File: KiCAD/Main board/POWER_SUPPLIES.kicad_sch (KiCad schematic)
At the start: 30 parts, among them U18 12V, U19 5V, U20 8V, U21 15V, U23 LIN_REG_±5V, U24 LIN_REG_±12V, U28 12V, U29 AP2111H-3.3TRG1, U31 AP2111H-3.3TRG1, U9 SEPIC_-15V_LT3579

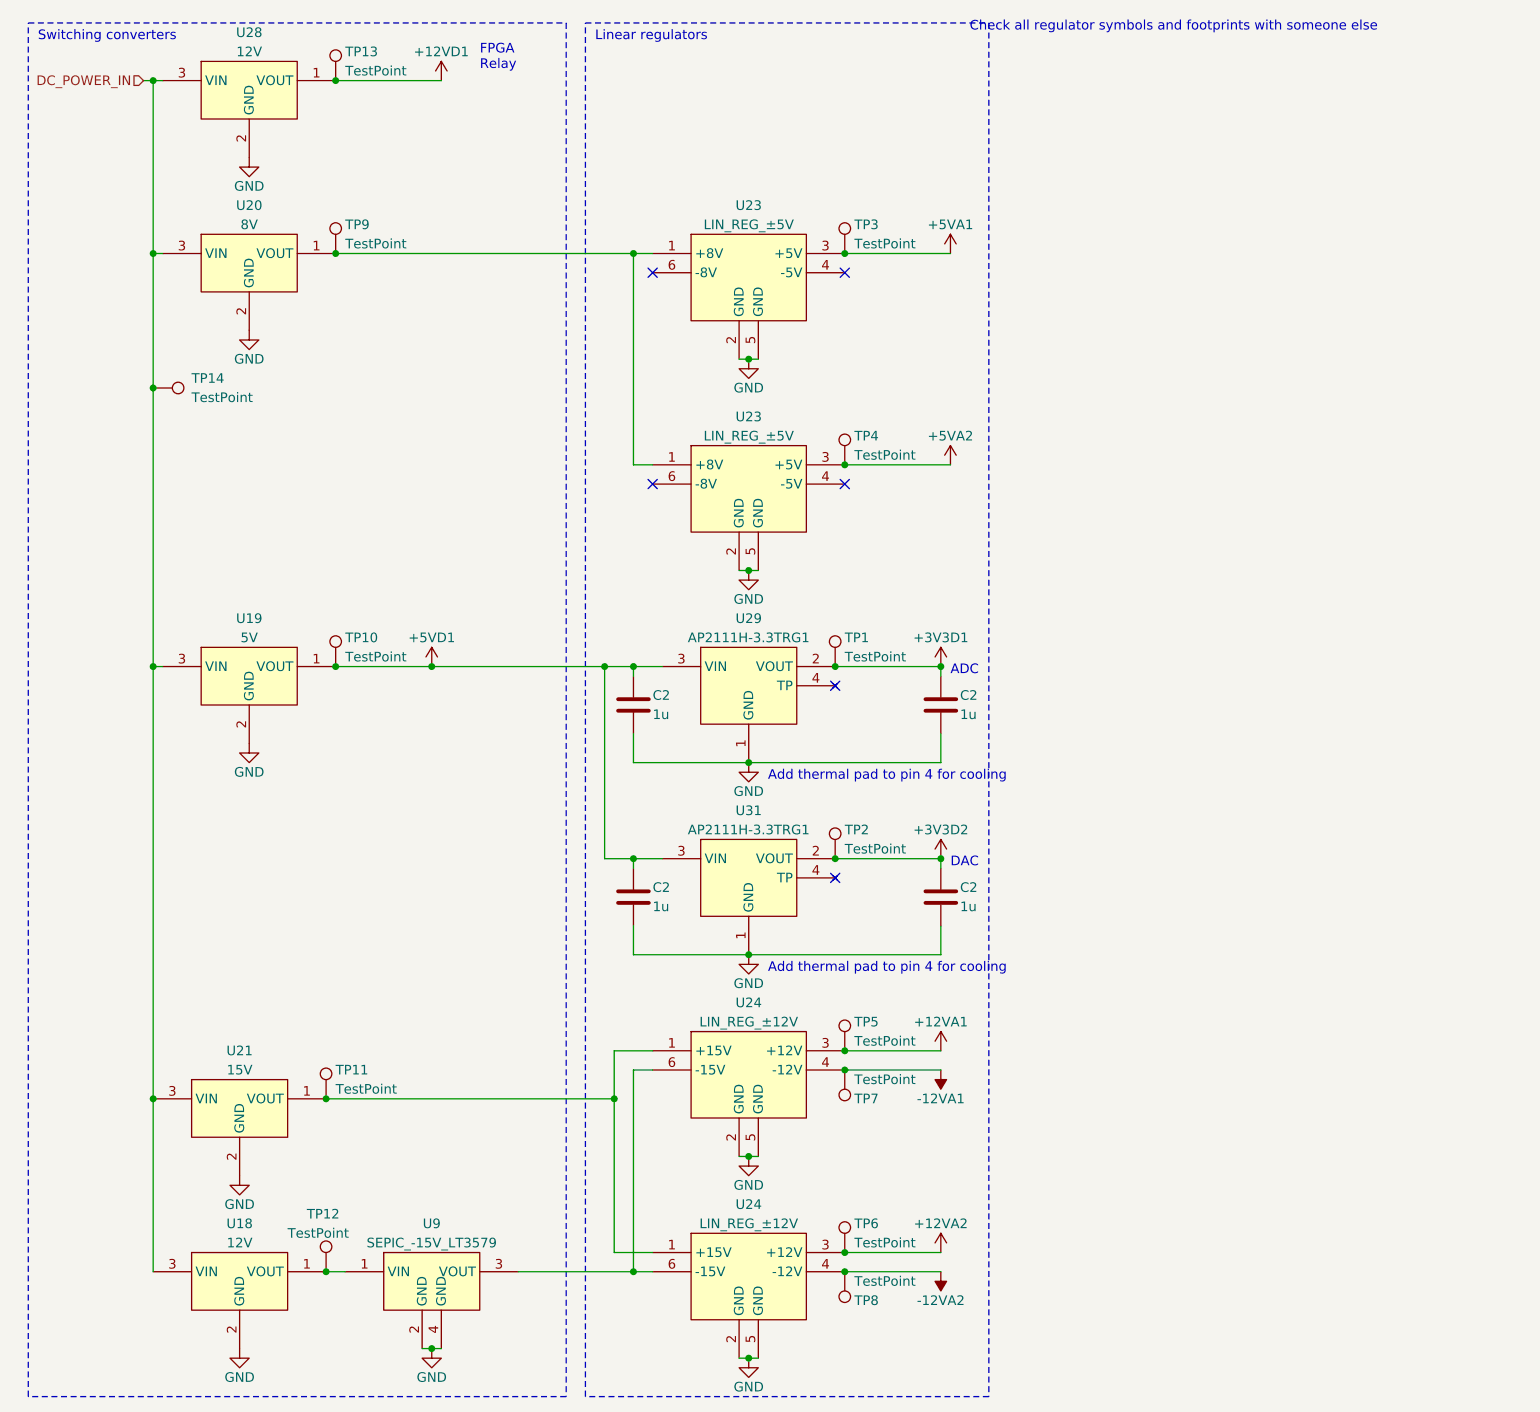
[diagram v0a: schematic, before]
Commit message: Worked in main board
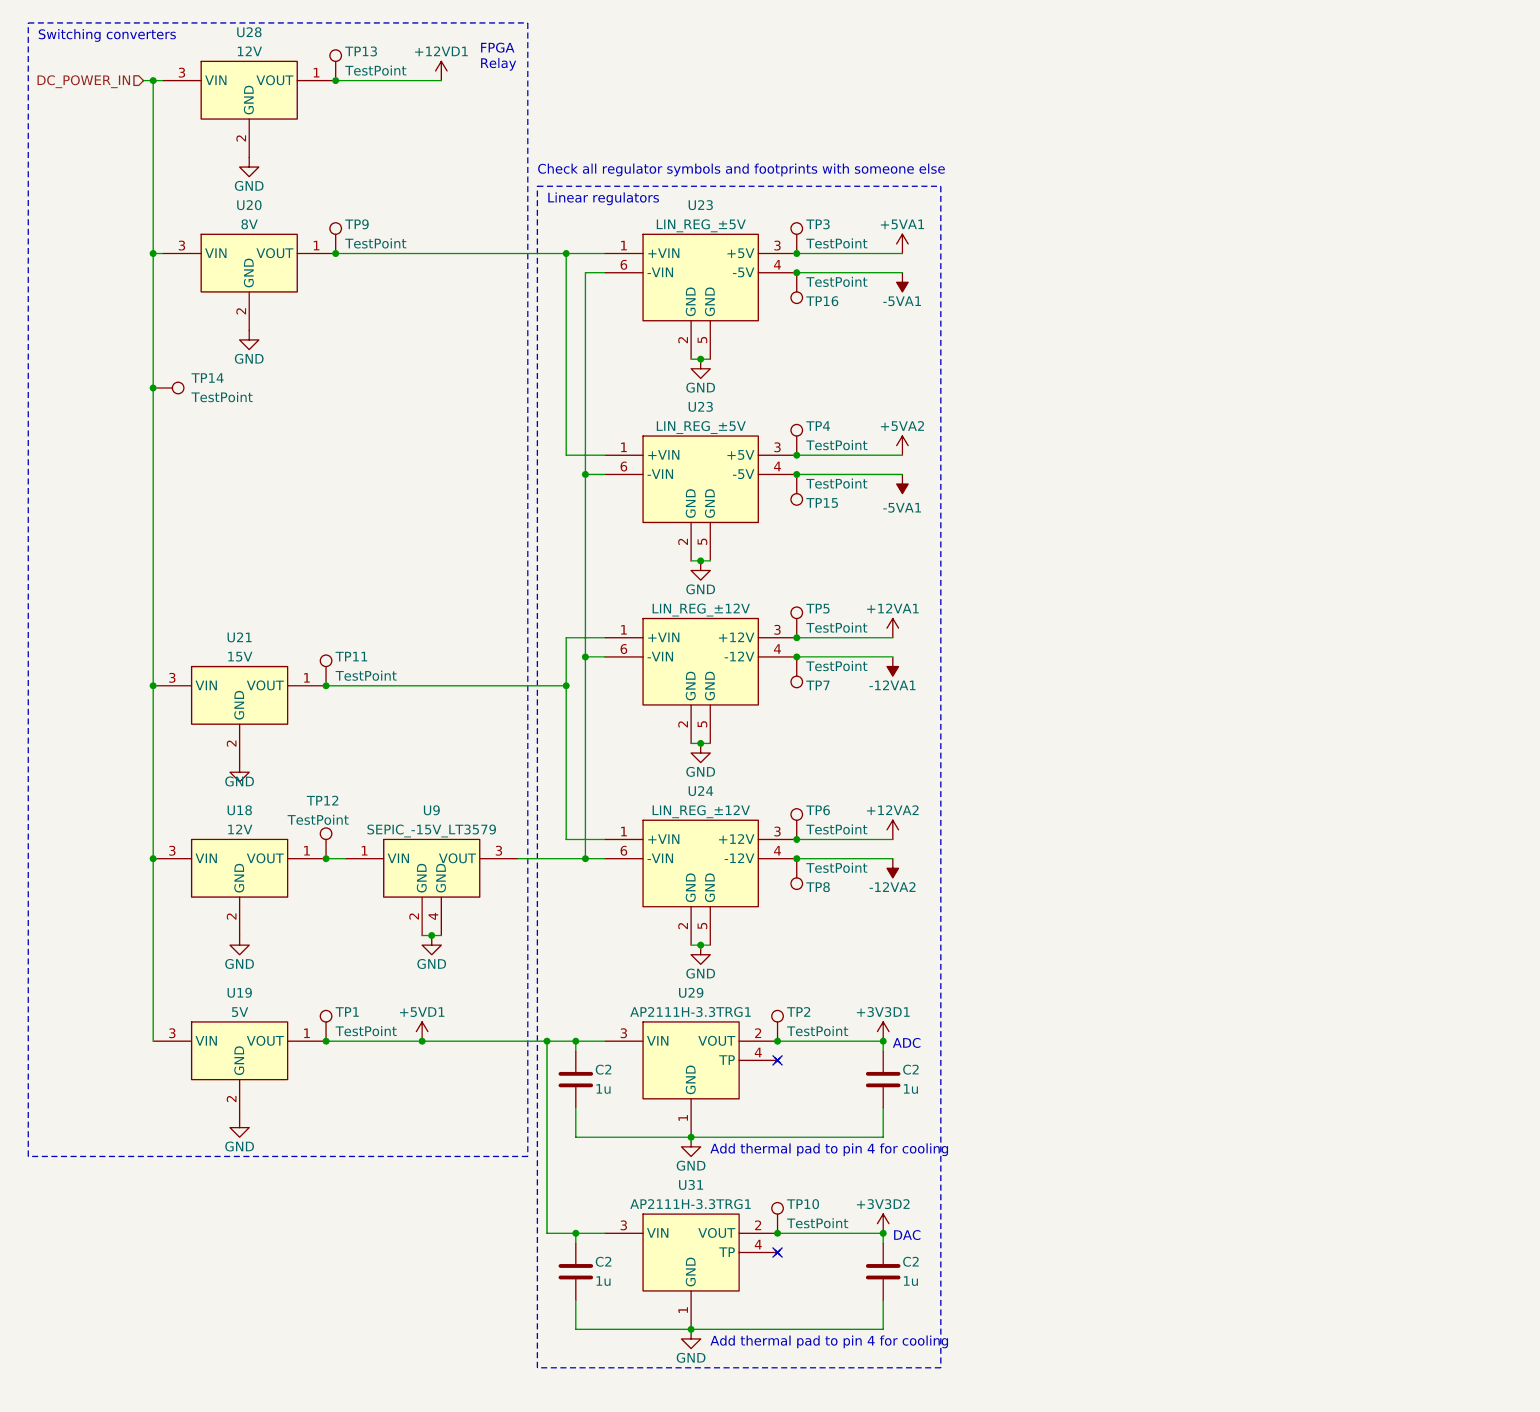
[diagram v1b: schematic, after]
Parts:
- removed C2 (x4): 1u, Capacitor_SMD:C_0402_1005Metric, symbol Device:C
- added C2 (x4): 1u, Capacitor_SMD:C_0402_1005Metric, symbol Device:C
- added TP15, TP16: TestPoint, TestPoint:TestPoint_Pad_D2.0mm, symbol Connector:TestPoint
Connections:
- net +3V3D1: now also TP2.1, C2.1; no longer TP1.1
- net +3V3D2: now also TP10.1, C2.1; no longer TP2.1
- net +5VD1: now also TP1.1, C2.1, C2.1; no longer TP10.1
- net GND: now also C2.2, C2.2, C2.2, C2.2
- net -5VA1: now reaches U23.4 (-5V)
- net -5VA1: now also U23.4 (-5V), TP15.1, TP16.1
- net at U23.6 (-VIN): now also U23.6 (-VIN), U24.6 (-VIN), U24.6 (-VIN), U9.3 (VOUT)
- no-connect marks 6 -> 2
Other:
- moved on the sheet: TP11, TP12, TP3, TP4, TP5, TP6, TP7, TP8, U18, U21, U23, U24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
